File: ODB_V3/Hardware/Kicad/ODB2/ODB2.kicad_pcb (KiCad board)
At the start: 4 copper layers, 63.5 x 127 mm, 241 parts, among them IC1 W25Q512JVEIQ, J1 1715310000, J10 GPS_Conn_02x04_Top_Bottom, J15 Vin_XT30PW-F, J2 RFD_GT17HN-4DP-2HA56, J3 SYS_SW_Conn_01x05_Header, J5 MEM2067, J6 IdeFIX_GT17HN-4DP-2HA56, J7 1715250000, J8 1715310000, J9 1715250000, U1 STM32F412ZGTx, U10 ADXL382-2BCCZ-RL7, U11 SI5442DU-T1-GE3, U12 SI5442DU-T1-GE3, U13 L6981N33DR, U2 LM339, U3 SI5442DU-T1-GE3, U4 MS580301BA01-00, U6 BNO055, U7 MPQ9843GLE-5-AEC1-Z, U8 SI5442DU-T1-GE3, U9 MAX6612MXK, Y1 ABM8G-25.000MHZ-18-D2Y-T

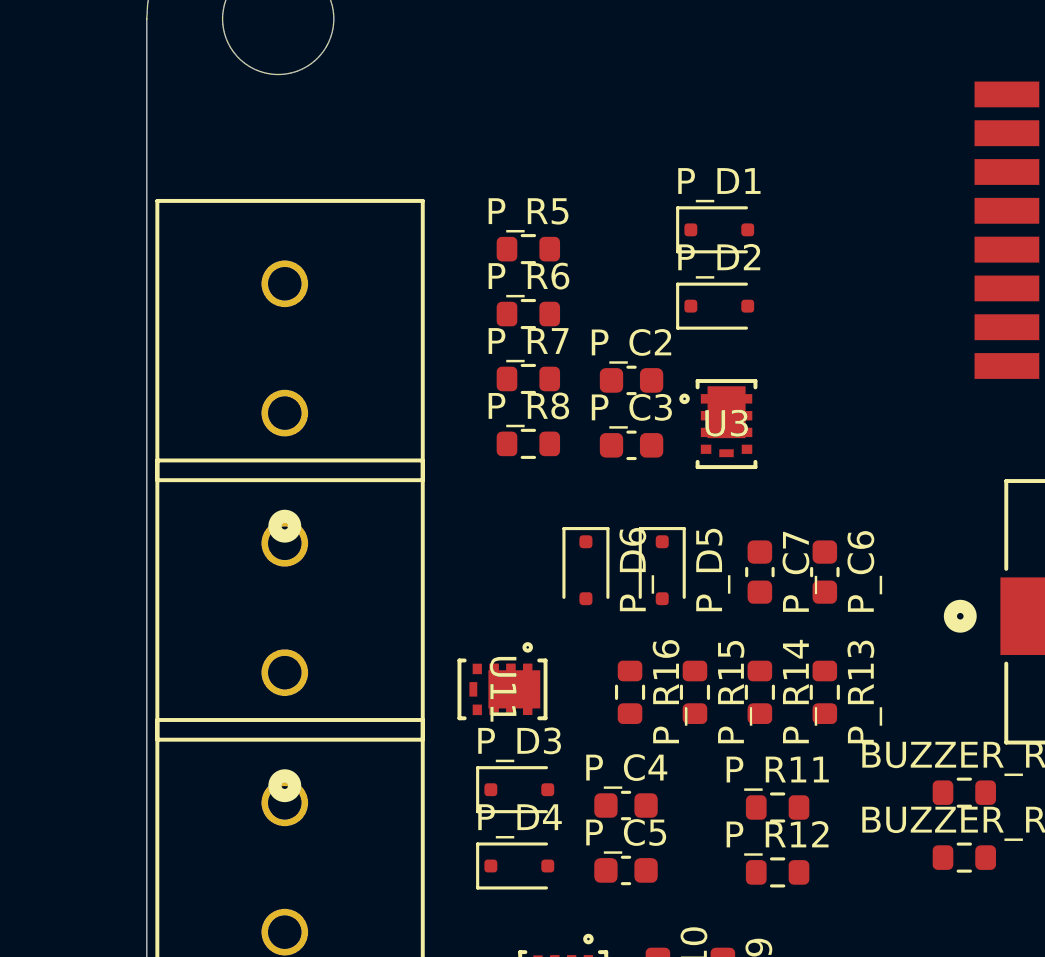
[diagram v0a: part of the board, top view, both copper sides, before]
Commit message: wip: pyro1 & pyro2
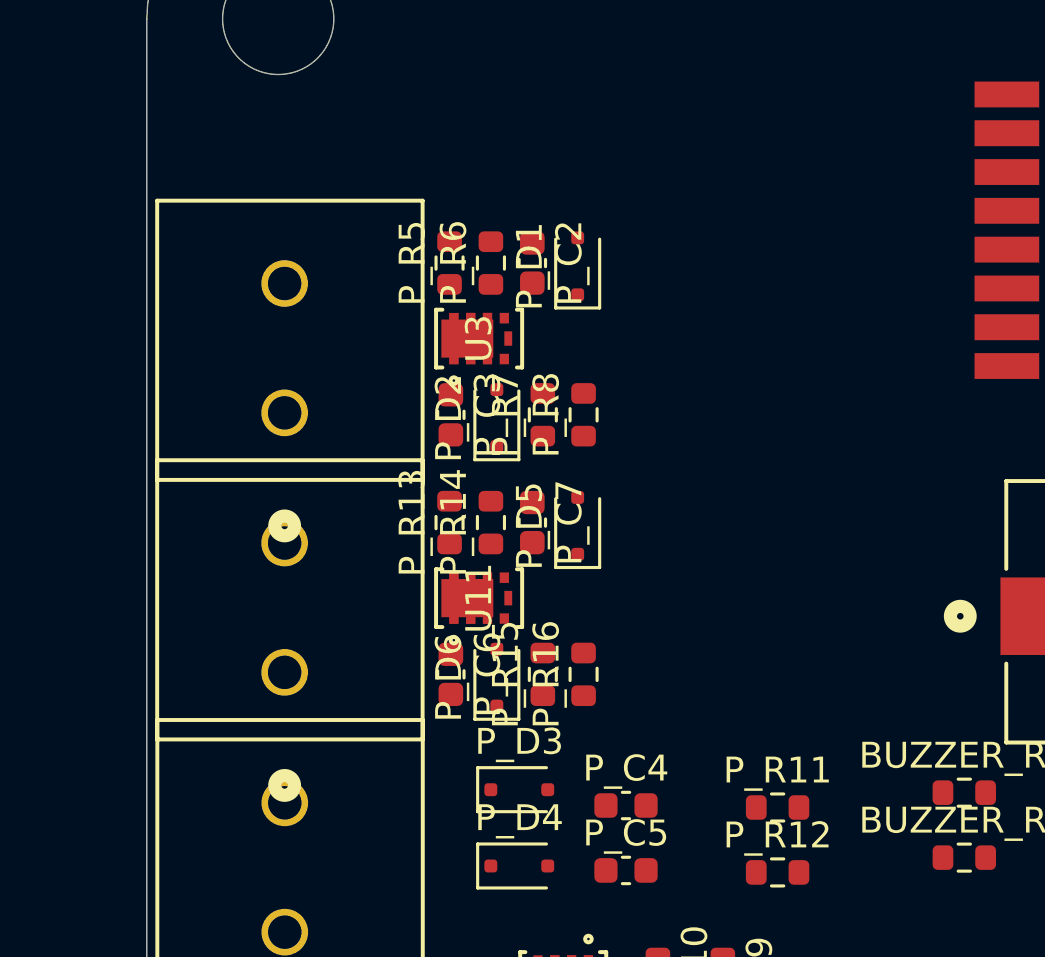
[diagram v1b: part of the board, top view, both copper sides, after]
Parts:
- moved P_R13 15.9 mm to (32.0, 44.6), turned to 90 degrees
- moved P_C6 15.0 mm to (32.0, 50.4)
- moved P_R14 12.3 mm to (33.6, 44.6), turned to 90 degrees
- moved U3 10.1 mm to (33.1, 37.4), turned to 90 degrees
- moved P_D2 9.63 mm to (33.8, 40.5), turned to 90 degrees
- moved P_C7 9.00 mm to (35.2, 44.6)
- moved P_C3 7.08 mm to (32.0, 40.4), turned to -90 degrees
- moved P_C2 5.94 mm to (35.2, 34.5), turned to -90 degrees
- moved P_R15 5.92 mm to (35.6, 50.4), turned to 90 degrees
- moved P_D1 5.65 mm to (36.9, 34.6), turned to 90 degrees
- moved P_D6 5.39 mm to (33.8, 50.5), turned to 90 degrees
- moved P_D5 3.69 mm to (36.9, 44.7), turned to 90 degrees
- moved U11 3.64 mm to (33.1, 47.5), turned to 90 degrees
- moved P_R5 3.09 mm to (32.0, 34.5), turned to 90 degrees
- moved P_R6 2.45 mm to (33.6, 34.5), turned to 90 degrees
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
